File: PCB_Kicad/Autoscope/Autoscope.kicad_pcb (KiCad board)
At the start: 2 copper layers, 85 x 56 mm, 42 parts, among them J1 Conn_01x02, J10 Conn_02x02_Odd_Even, J11 Conn_02x02_Odd_Even, J12 Conn_02x02_Odd_Even, J13 Conn_01x02, J2 Conn_01x02, J3 Conn_01x02, J4 Conn_01x02, J5 Conn_01x02, J6 12VDC Supply, J7 Conn_01x04, J8 Conn_02x20_Odd_Even, J9 Conn_01x05, SW1 Conn_01x02, U1 R-78B5.0-2.0, U2 A4988, U3 A4988, U4 A4988

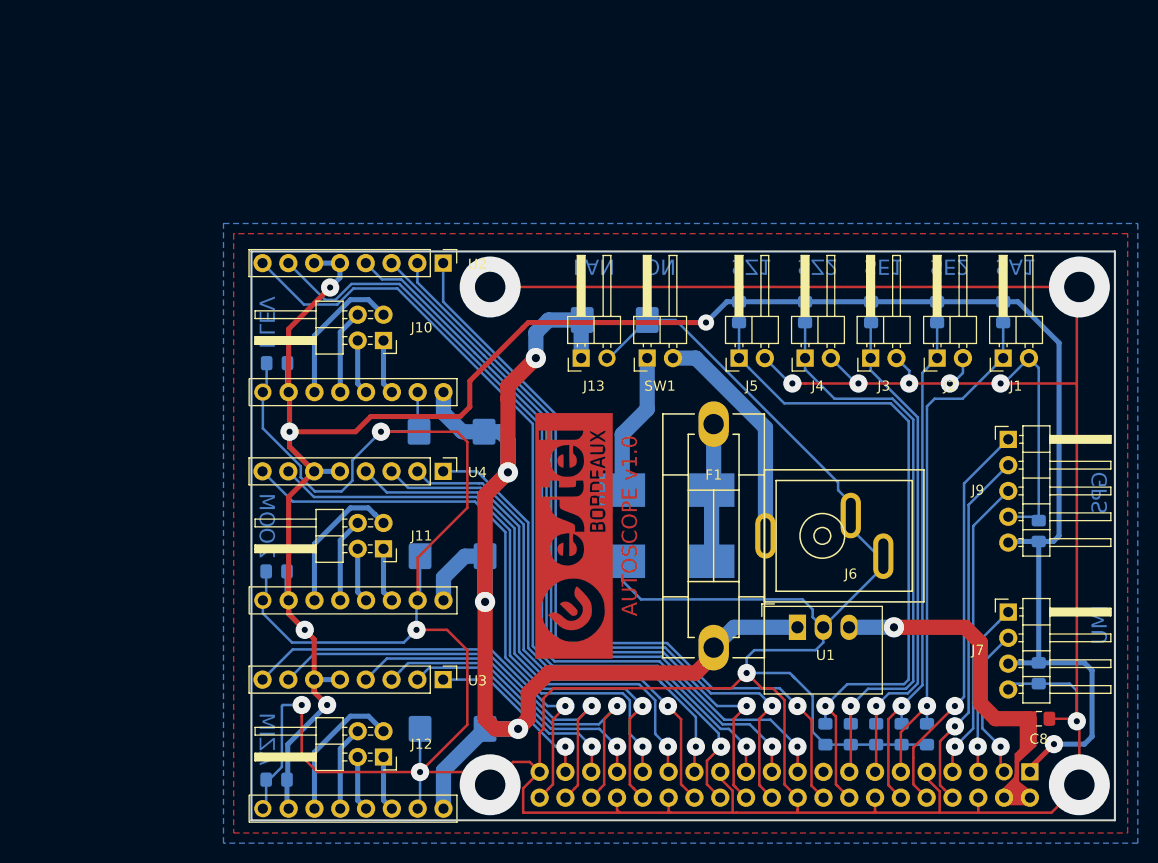
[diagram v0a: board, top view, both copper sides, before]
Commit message: add A5 fab files
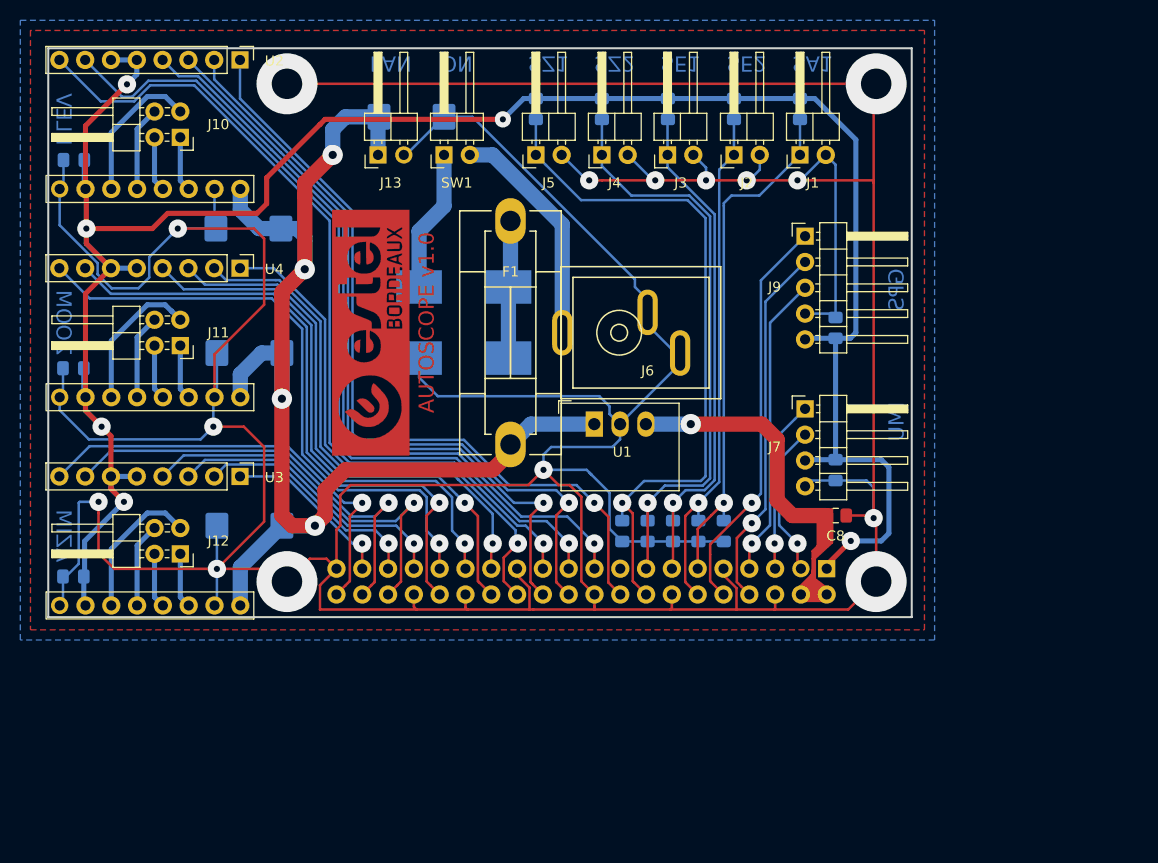
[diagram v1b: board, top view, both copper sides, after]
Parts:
- moved C12 28.3 mm to (62.5, 41.0)
- moved C7 28.3 mm to (137.5, 57.5)
- moved J3 28.3 mm to (121.0, 40.5)
- moved C1 28.3 mm to (126.5, 77.5)
- moved C10 28.3 mm to (79.8, 60.0)
- moved C11 28.3 mm to (79.8, 77.0)
- moved C15 28.3 mm to (95.8, 36.8)
- moved C2 28.3 mm to (124.0, 77.5)
- moved C3 28.3 mm to (121.5, 77.5)
- moved C4 28.3 mm to (119.0, 77.5)
- moved C5 28.3 mm to (116.5, 77.5)
- moved C6 28.3 mm to (137.5, 71.5)
- moved C8 28.3 mm to (137.5, 76.0)
- moved C9 28.3 mm to (79.7, 47.8)
- moved D1 28.3 mm to (100.9, 53.5)
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
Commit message: Revert "add A5 fab files"
This reverts commit e4fdc3836b1555d306f2fe8898c2b94182f1870a.
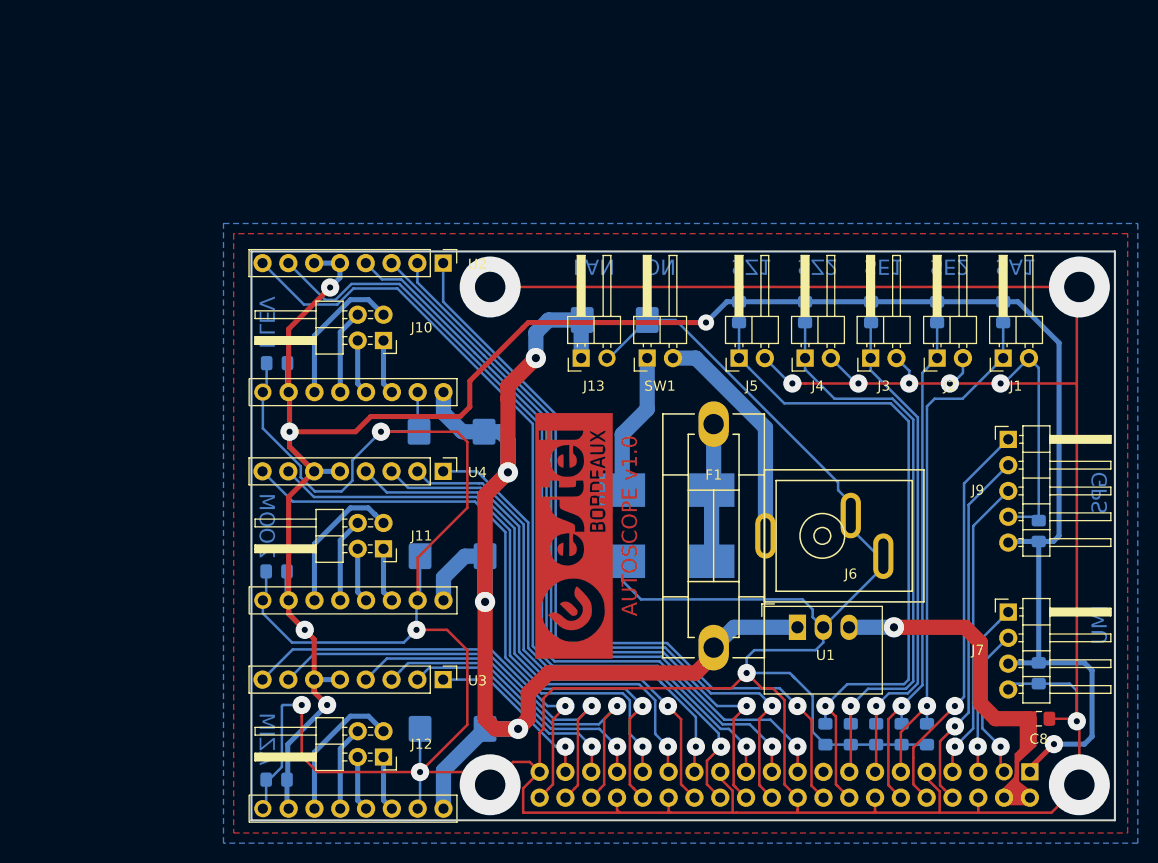
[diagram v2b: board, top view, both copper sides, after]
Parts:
- moved C12 28.3 mm to (82.5, 61.0)
- moved C7 28.3 mm to (157.5, 77.5)
- moved J3 28.3 mm to (141.0, 60.5)
- moved C1 28.3 mm to (146.5, 97.5)
- moved C10 28.3 mm to (99.8, 80.0)
- moved C11 28.3 mm to (99.8, 97.0)
- moved C15 28.3 mm to (115.8, 56.8)
- moved C2 28.3 mm to (144.0, 97.5)
- moved C3 28.3 mm to (141.5, 97.5)
- moved C4 28.3 mm to (139.0, 97.5)
- moved C5 28.3 mm to (136.5, 97.5)
- moved C6 28.3 mm to (157.5, 91.5)
- moved C8 28.3 mm to (157.5, 96.0)
- moved C9 28.3 mm to (99.7, 67.8)
- moved D1 28.3 mm to (120.9, 73.5)
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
